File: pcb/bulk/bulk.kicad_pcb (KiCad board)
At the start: 2 copper layers, 75 x 65 mm, 94 parts

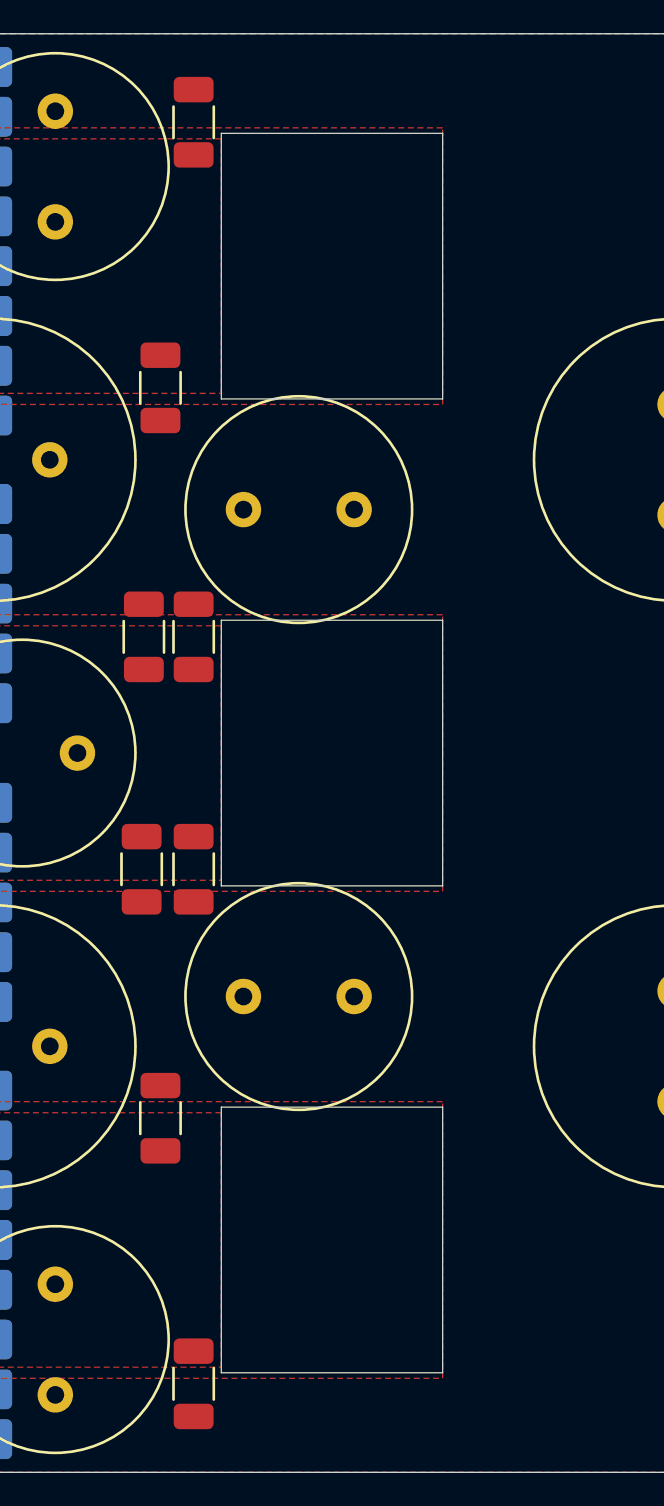
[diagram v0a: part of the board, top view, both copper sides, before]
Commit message: Save progress
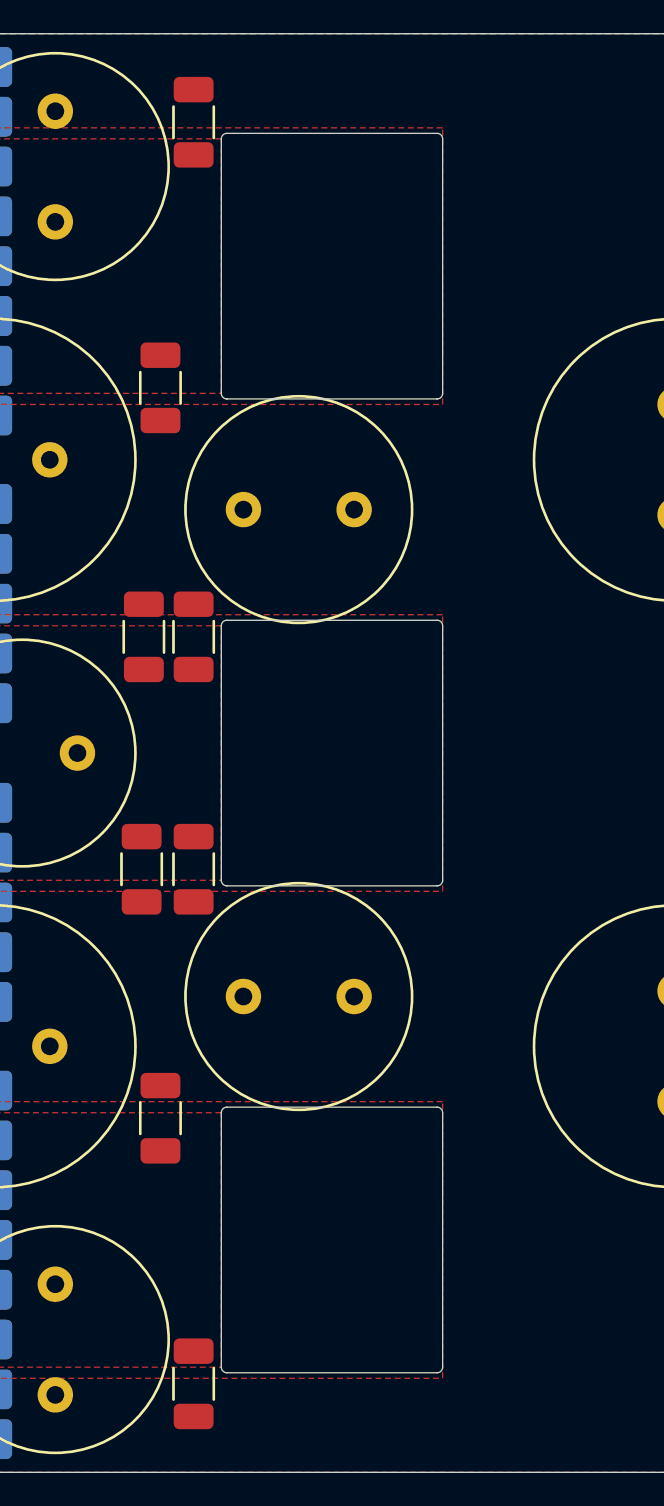
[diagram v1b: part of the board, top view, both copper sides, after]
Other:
- outline, holes or cut-outs redrawn
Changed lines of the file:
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@@
+	)
+	(gr_line
+		(start 59.000001 66.250001)
+		(end 59.000001 77.750001)
+		(stroke
+			(width 0.05)
+			(type default)
+		)
+		(layer "Edge.Cuts")
+	)
+	(gr_line
+		(start 59 22.25)
+		(end 59 33.75)
+		(stroke
+			(width 0.05)
+			(type default)
+		)
+		(layer "Edge.Cuts")
 	)
 	(gr_line
 		(start 100 19.999999)
 		(end 100 25.5)
+		(stroke
+			(width 0.05)
+			(type default)
+		)
+		(layer "Edge.Cuts")
+	)
+	(gr_line
+		(start 59.000001 44.250001)
+		(end 59.000001 55.750001)
+		(stroke
+			(width 0.05)
+			(type default)
+		)
+		(layer "Edge.Cuts")
+	)
+	(gr_line
+		(start 69 22.25)
+		(end 69 33.75)
 		(stroke
 			(width 0.05)
@@
 		(layer "Edge.Cuts")
 	)
-	(gr_rect
-		(start 59 22)
-		(end 69 34)
-		(stroke
-			(width 0.05)
-			(type default)
-		)
-		(fill no)
-		(layer "Edge.Cuts")
-	)
 	(gr_line
 		(start 27.5 82.5)
@@
 		(layer "Edge.Cuts")
 	)
-	(gr_rect
-		(start 59 44)
-		(end 69 56)
-		(stroke
-			(width 0.05)
-			(type default)
-		)
-		(fill no)
+	(gr_line
+		(start 69.000001 66.250001)
+		(end 69.000001 77.750001)
+		(stroke
+			(width 0.05)
+			(type default)
+		)
 		(layer "Edge.Cuts")
 	)
@@
 		(layer "Edge.Cuts")
 	)
-	(gr_rect
-		(start 59 66)
-		(end 69 78)
-		(stroke
-			(width 0.05)
-			(type default)
-		)
-		(fill no)
+	(gr_arc
+		(start 59.000001 66.250001)
+		(mid 59.073224 66.073224)
+		(end 59.250001 66.000001)
+		(stroke
+			(width 0.05)
+			(type default)
+		)
+		(layer "Edge.Cuts")
+	)
+	(gr_arc
+		(start 69.000001 77.750001)
+		(mid 68.926778 77.926778)
+		(end 68.750001 78.000001)
+		(stroke
+			(width 0.05)
+			(type default)
+		)
+		(layer "Edge.Cuts")
+	)
+	(gr_line
+		(start 68.75 34)
+		(end 59.25 34)
+		(stroke
+			(width 0.05)
+			(type default)
+		)
+		(layer "Edge.Cuts")
+	)
+	(gr_line
+		(start 69.000001 44.250001)
+		(end 69.000001 55.750001)
+		(stroke
+			(width 0.05)
+			(type default)
+		)
+		(layer "Edge.Cuts")
+	)
+	(gr_arc
+		(start 69 33.75)
+		(mid 68.926777 33.926777)
+		(end 68.75 34)
+		(stroke
+			(width 0.05)
+			(type default)
+		)
+		(layer "Edge.Cuts")
+	)
+	(gr_arc
+		(start 59.25 34)
+		(mid 59.073223 33.926777)
+		(end 59 33.75)
+		(stroke
+			(width 0.05)
+			(type default)
+		)
+		(layer "Edge.Cuts")
+	)
+	(gr_line
+		(start 59.25 22)
+		(end 68.75 22)
+		(stroke
+			(width 0.05)
+			(type default)
+		)
+		(layer "Edge.Cuts")
+	)
+	(gr_line
+		(start 68.750001 56.000001)
+		(end 59.250001 56.000001)
+		(stroke
+			(width 0.05)
+			(type default)
+		)
+		(layer "Edge.Cuts")
+	)
+	(gr_arc
+		(start 68.750001 66.000001)
+		(mid 68.926778 66.073224)
+		(end 69.000001 66.250001)
+		(stroke
+			(width 0.05)
+			(type default)
+		)
 		(layer "Edge.Cuts")
 	)
@@
 		(layer "Edge.Cuts")
 	)
+	(gr_arc
+		(start 59.250001 78.000001)
+		(mid 59.073224 77.926778)
+		(end 59.000001 77.750001)
+		(stroke
+			(width 0.05)
+			(type default)
+		)
+		(layer "Edge.Cuts")
+	)
+	(gr_arc
+		(start 59.000001 44.250001)
+		(mid 59.073224 44.073224)
+		(end 59.250001 44.000001)
+		(stroke
+			(width 0.05)
+			(type default)
+		)
+		(layer "Edge.Cuts")
+	)
 	(gr_line
 		(start 100 52.5)
@@
 		(start 100 74.5)
 		(end 100 80)
+		(stroke
+			(width 0.05)
+			(type default)
+		)
+		(layer "Edge.Cuts")
+	)
+	(gr_line
+		(start 59.250001 66.000001)
+		(end 68.750001 66.000001)
+		(stroke
+			(width 0.05)
+			(type default)
+		)
+		(layer "Edge.Cuts")
+	)
+	(gr_arc
+		(start 68.750001 44.000001)
+		(mid 68.926778 44.073224)
+		(end 69.000001 44.250001)
+		(stroke
+			(width 0.05)
+			(type default)
+		)
+		(layer "Edge.Cuts")
+	)
+	(gr_arc
+		(start 69.000001 55.750001)
+		(mid 68.926778 55.926778)
+		(end 68.750001 56.000001)
+		(stroke
+			(width 0.05)
+			(type default)
+		)
+		(layer "Edge.Cuts")
+	)
+	(gr_arc
+		(start 59.250001 56.000001)
+		(mid 59.073224 55.926778)
+		(end 59.000001 55.750001)
 		(stroke
 			(width 0.05)
@@
 	)
 	(gr_line
+		(start 59.250001 44.000001)
+		(end 68.750001 44.000001)
+		(stroke
+			(width 0.05)
+			(type default)
+		)
+		(layer "Edge.Cuts")
+	)
+	(gr_line
 		(start 97.5 17.5)
 		(end 27.5 17.5)
+		(stroke
+			(width 0.05)
+			(type default)
+		)
+		(layer "Edge.Cuts")
+	)
+	(gr_arc
+		(start 68.75 22)
+		(mid 68.926777 22.073223)
+		(end 69 22.25)
 		(stroke
 			(width 0.05)
@@
 	)
 	(gr_line
+		(start 68.750001 78.000001)
+		(end 59.250001 78.000001)
+		(stroke
+			(width 0.05)
+			(type default)
+		)
+		(layer "Edge.Cuts")
+	)
+	(gr_line
 		(start 25 69.5)
 		(end 25 52.5)
 		(stroke
 			(width 0.05)
+			(type default)
+		)
+		(layer "Edge.Cuts")
+	)
+	(gr_arc
+		(start 59 22.25)
+		(mid 59.073223 22.073223)
+		(end 59.25 22)
+		(stroke
+			(width 0.05)
